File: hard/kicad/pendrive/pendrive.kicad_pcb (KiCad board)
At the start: 2 copper layers, 8 parts, among them J1 IOx, U1 62256, U2 74HC138, U3 74HC574, U4 74HC574

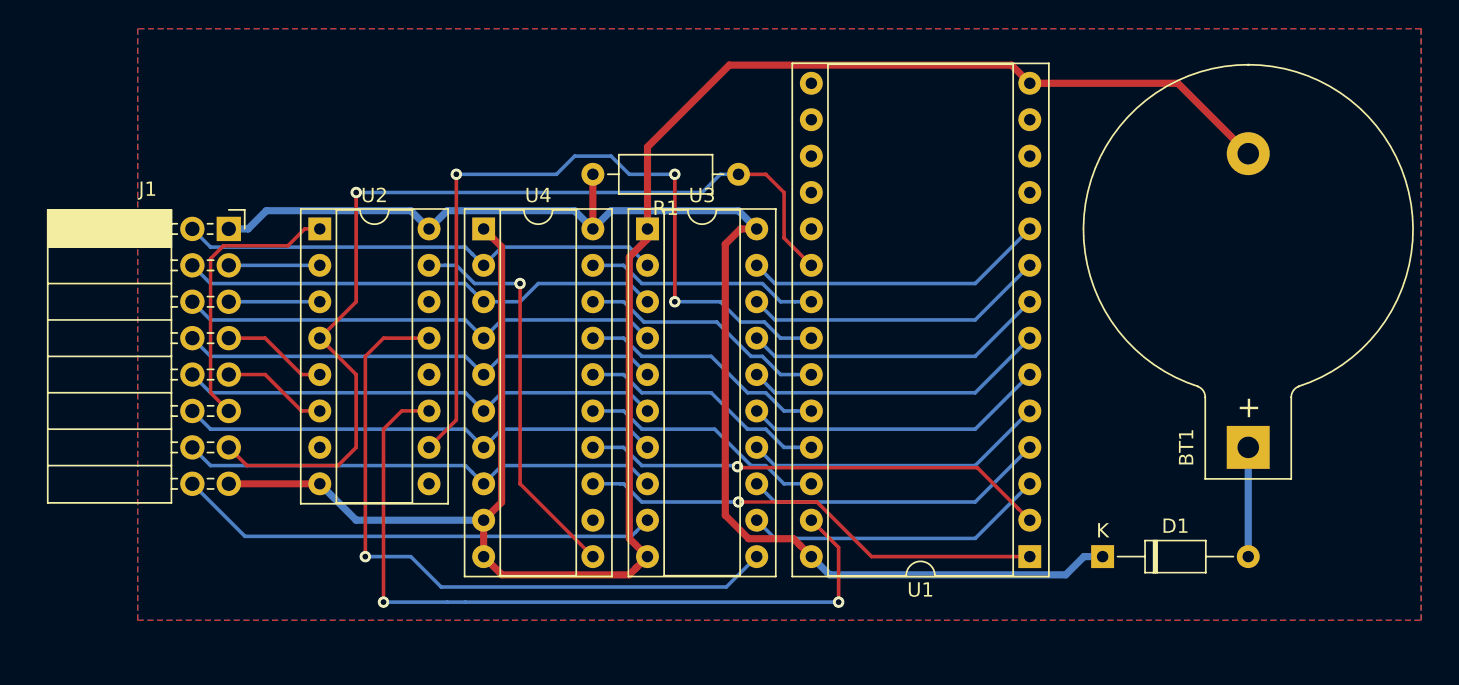
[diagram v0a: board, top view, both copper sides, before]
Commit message: retraced pendrive
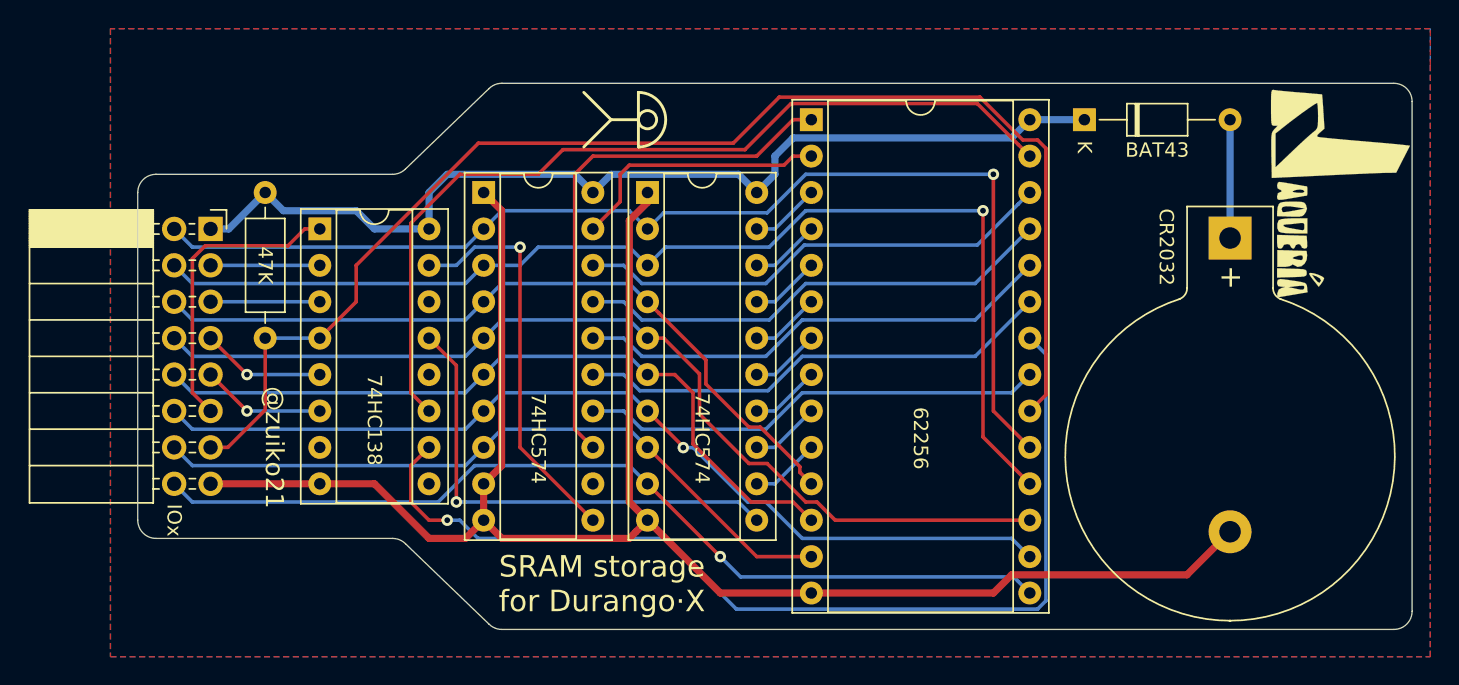
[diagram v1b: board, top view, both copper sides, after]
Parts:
- added LOGO1: Logo_Open_Hardware_Small, durango:jaqueria, F.Cu at (245.1, 34.3)
- added LOGO2: Logo_Open_Hardware_Large, Symbol:OSHW-Logo_19x20mm_SilkScreen, B.Cu at (238.1, 48.3)
- D1: value D_Schottky -> BAT43
- moved R1 34.9 mm to (170.2, 44.5), turned to 90 degrees
- moved U1 34.1 mm to (208.3, 29.2), turned to 0 degrees
- moved D1 30.5 mm to (227.3, 29.2)
- moved BT1 14.7 mm to (237.5, 37.5), turned to 270 degrees
- moved U3 2.54 mm to (196.8, 34.3)
- moved U4 2.54 mm to (185.4, 34.3)
- moved J1 1.27 mm to (166.4, 36.8)
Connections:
- U1 pad 10: /A0 -> /A7
- U1 pad 12: /PD1 -> /PD4
- U1 pad 13: /PD0 -> /PD6
- U1 pad 15: /PD3 -> /PD7
- U1 pad 16: /PD4 -> /PD5
- U1 pad 17: /PD5 -> /PD3
- U1 pad 18: /PD6 -> /PD1
- U1 pad 19: /PD7 -> /PD0
- U1 pad 2: /A13 -> /A8
- U1 pad 21: /A8 -> /A13
- U1 pad 23: /A9 -> /A12
- U1 pad 24: /A10 -> /A11
- U1 pad 25: /A11 -> /A10
- U1 pad 26: /A12 -> /A9
- U1 pad 3: /A7 -> /A0
- U1 pad 4: /A6 -> /A1
- U1 pad 5: /A5 -> /A2
- U1 pad 6: /A4 -> /A3
- U1 pad 7: /A3 -> /A4
- U1 pad 8: /A2 -> /A5
- U1 pad 9: /A1 -> /A6
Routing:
- net /PD0: track 33.9 -> 80.9 mm, vias 0 -> 1
- net /PD1: track 33.9 -> 80.5 mm, vias 0 -> 1
- net /PD3: track 33.9 -> 68.7 mm
- net /PD5: track 33.9 -> 66.0 mm, vias 0 -> 1
- net /PD7: track 33.7 -> 65.0 mm, vias 0 -> 1
- net /~IOX: track 66.6 -> 93.1 mm, vias 1 -> 0
- net +5V: track 93.9 -> 70.6 mm
- net /PD2: track 33.9 -> 53.0 mm
- net /PD4: track 33.9 -> 52.9 mm
- net /A10: track 17.3 -> 33.6 mm
- net /A9: track 17.3 -> 33.6 mm
- net /A11: track 17.3 -> 33.6 mm
- net /A7: track 21.2 -> 4.86 mm
- net /A6: track 21.2 -> 4.86 mm
- net /A5: track 21.2 -> 4.86 mm
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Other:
- board outline added: 88.9 x 38.1 mm
- board text added: "@zuiko21"
- board text added: "SRAM storage for Durango·X"
- board text added: "https://www.durangoretro.com"
